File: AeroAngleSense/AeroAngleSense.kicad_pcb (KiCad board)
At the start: 2 copper layers, 15 x 55 mm, 23 parts, among them J1 SM06B-GHS-TBT, J2 SM04B-GHS-TBT, U1 STM32F042F6P6, U2 TPS62842DGRR, U3 TMP127EDBVRQ1

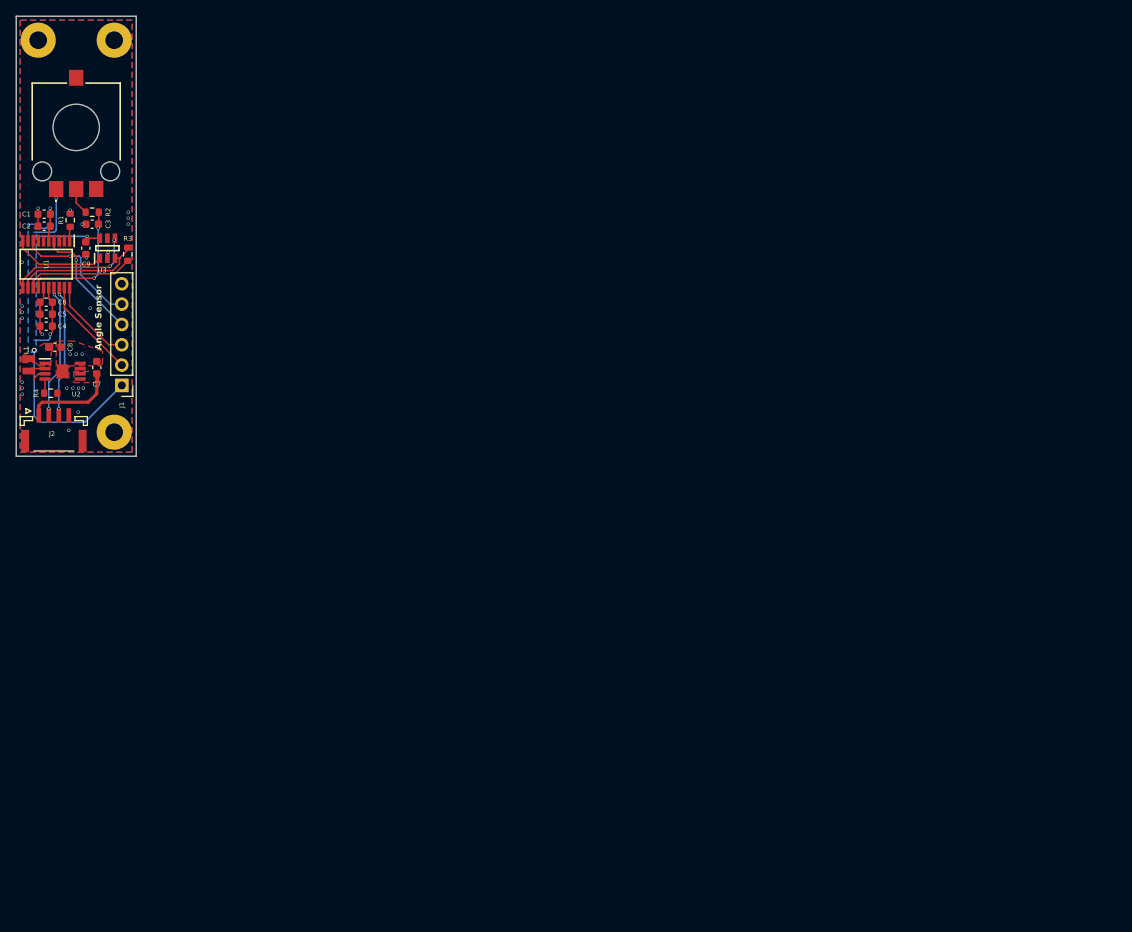
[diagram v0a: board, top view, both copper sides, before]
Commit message: fix:readme
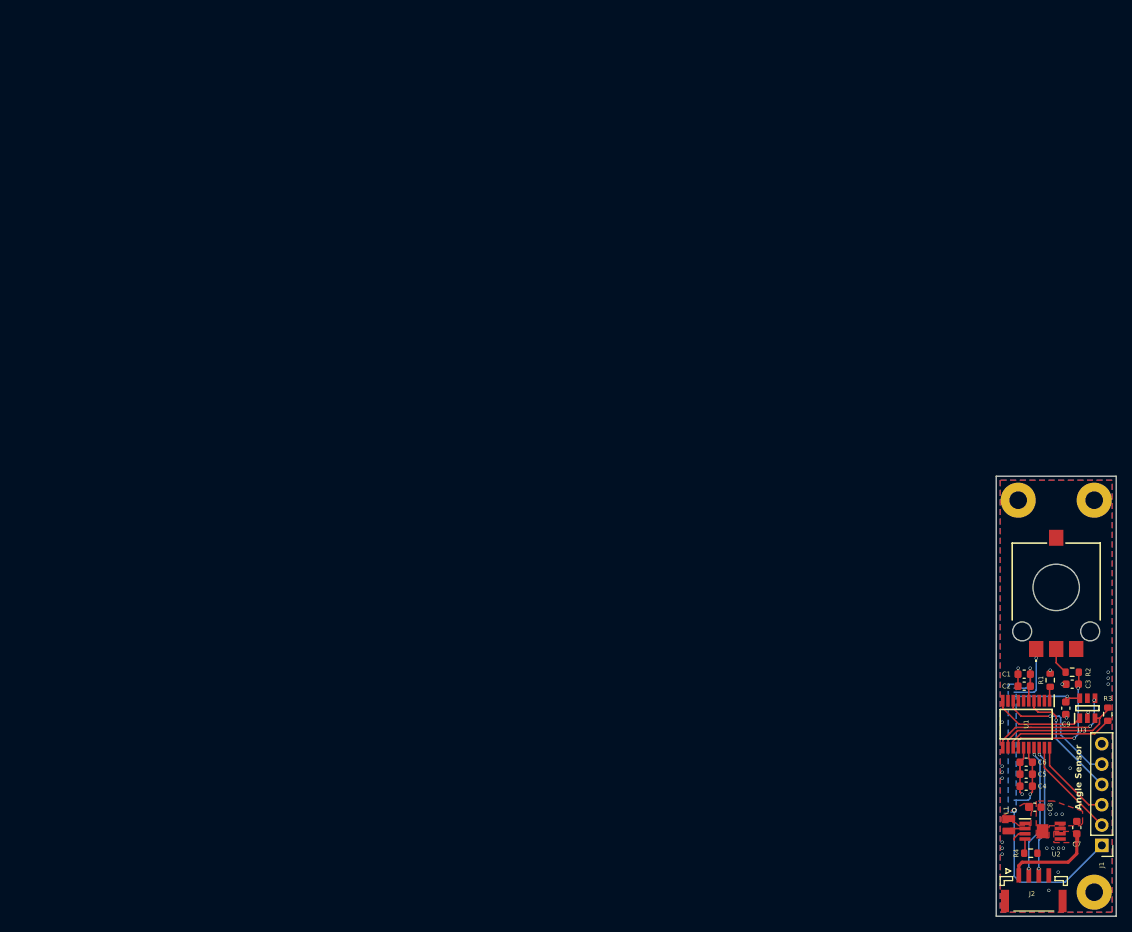
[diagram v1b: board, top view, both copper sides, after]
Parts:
- J1: value SM06B-GHS-TBT -> pinheader 2.54 6P
- moved U2 135.3 mm to (148.3, 116.9)
- moved C1 135.3 mm to (146.0, 97.2)
- moved C2 135.3 mm to (146.0, 98.8)
- moved C3 135.3 mm to (152.0, 98.5)
- moved C4 135.3 mm to (146.2, 111.2)
- moved C5 135.3 mm to (146.2, 109.8)
- moved C6 135.3 mm to (146.2, 108.2)
- moved C7 135.3 mm to (152.6, 116.4)
- moved C8 135.3 mm to (147.3, 113.9)
- moved C9 135.3 mm to (151.2, 101.5)
- moved H1 135.3 mm to (150.0, 86.9)
- moved H2 135.3 mm to (145.2, 75.5)
- moved H3 135.3 mm to (154.8, 75.5)
- moved H4 135.3 mm to (154.8, 124.5)
- moved J1 135.3 mm to (155.7, 118.7)
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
